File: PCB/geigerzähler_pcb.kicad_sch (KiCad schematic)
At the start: 95 parts, among them J1 Molex Micro Fit, J2 Debugpins, J3 USB-TYPE-C-018, J4 Femal Connector for LCD I2C b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, Q1 IRLML6402TRPBF, Q2 BCW68, Q3 PBHV8560Z, Q4 MMBT3904, Q5 MMBT3904, SW1 GPIO4, SW2 GPIO5, SW3 Reset, SW4 Boot, SW5 SW_SPDT, U1 TPS631000DRLR, U2 MCP73871-2AA, U3 ESP32-S3-WROOM-1_multi_unit, U4 ICM7555IBAZ

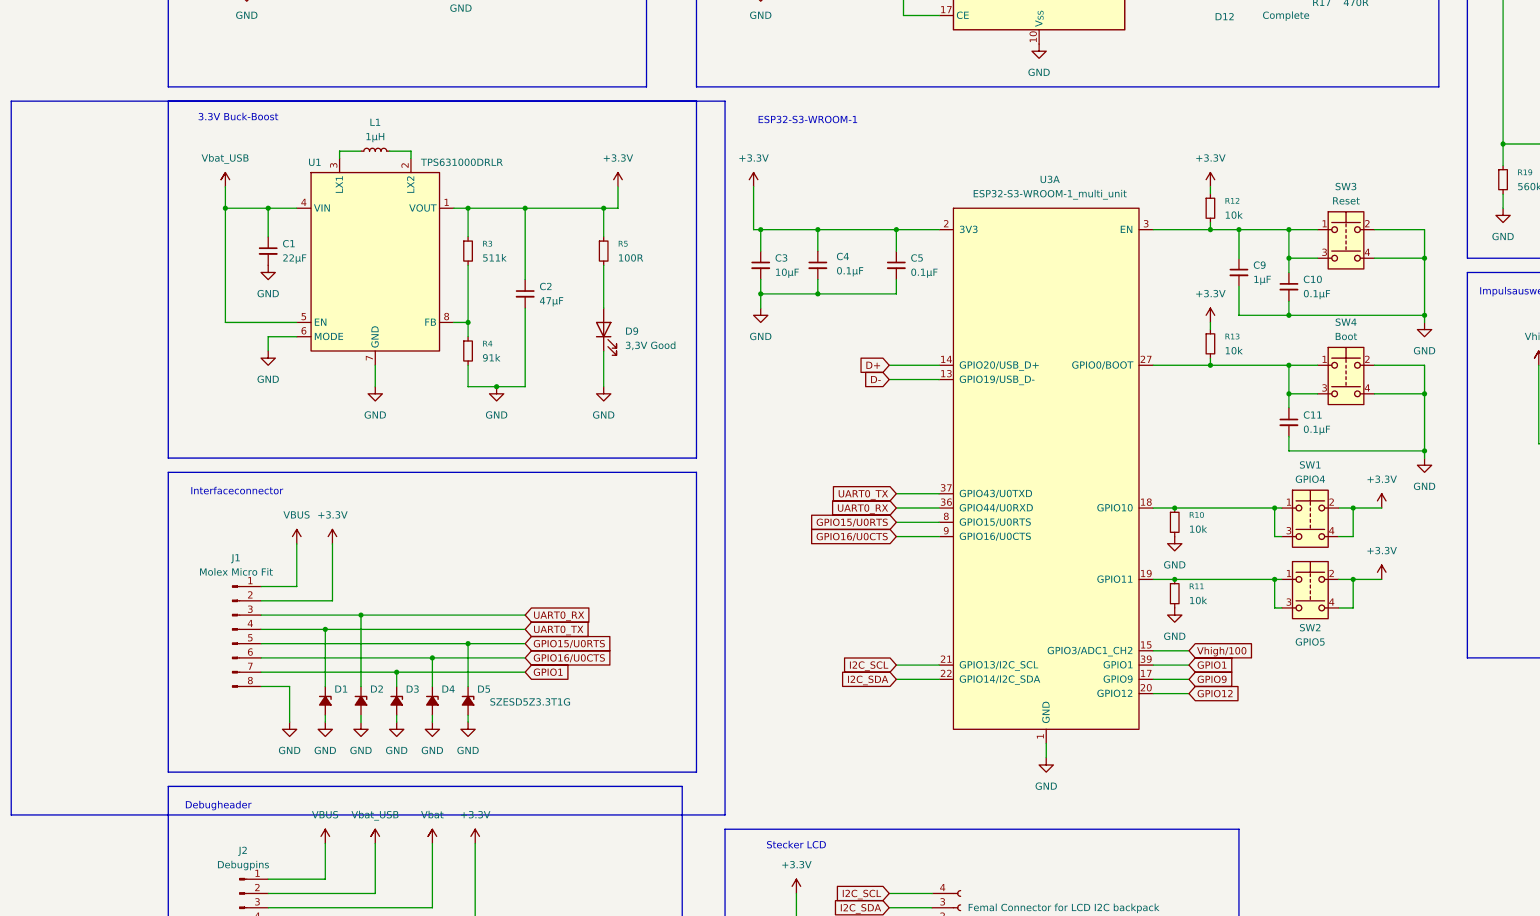
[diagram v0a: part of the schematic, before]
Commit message: 08.08.2025
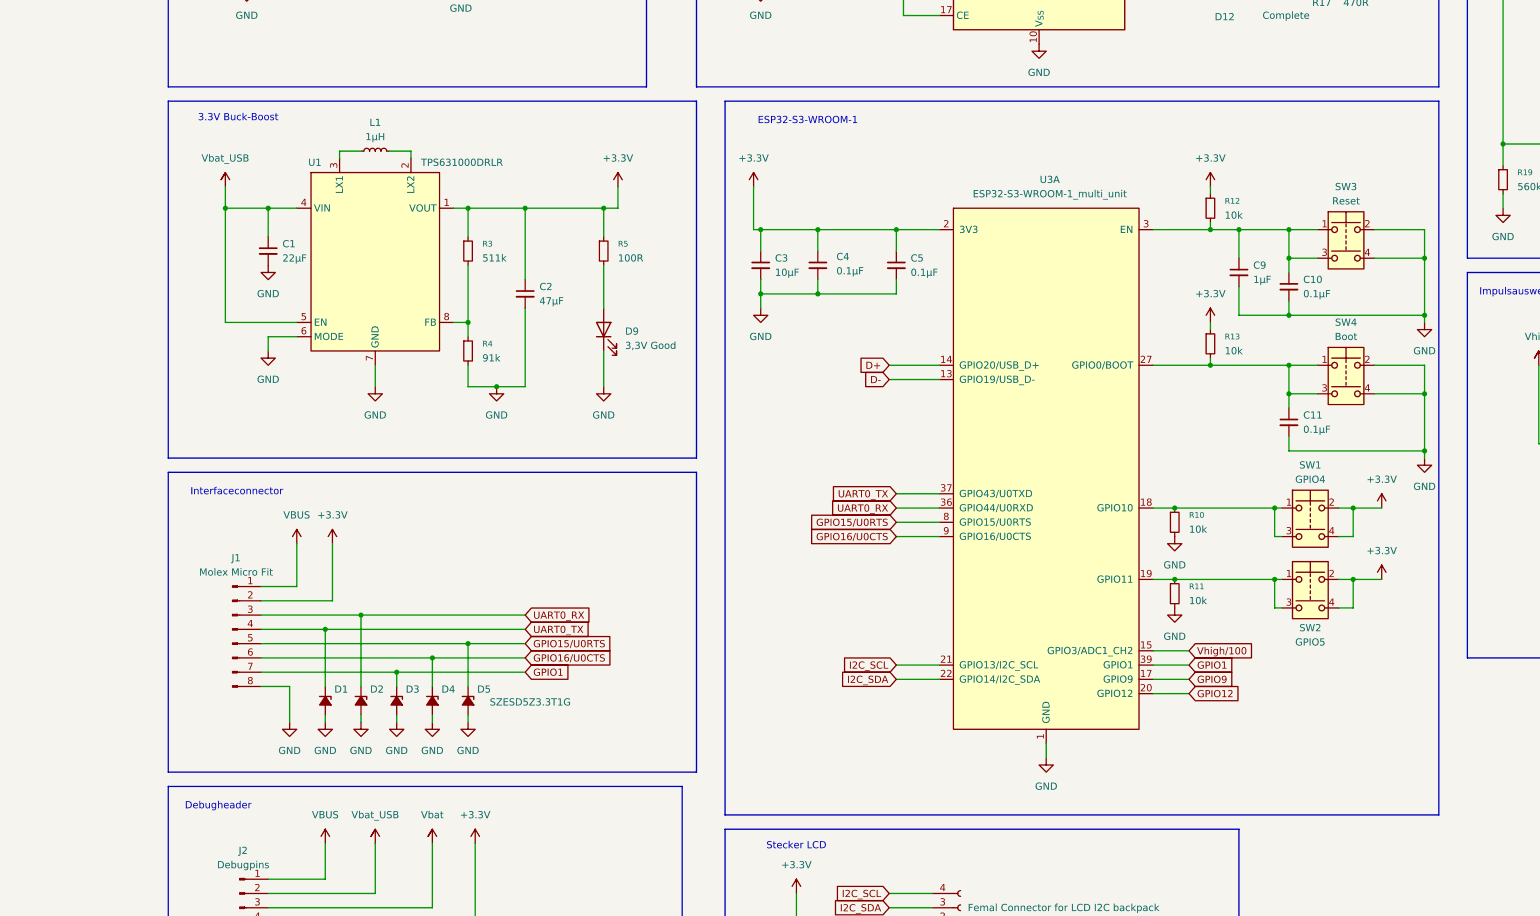
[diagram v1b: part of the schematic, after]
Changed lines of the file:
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@@
 	(rectangle
 		(start 114.3 93.98)
-		(end -12.7 220.98)
+		(end 241.3 220.98)
 		(stroke
 			(width 0)
